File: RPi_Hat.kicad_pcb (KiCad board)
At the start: 2 copper layers, 65 x 56.5 mm, 21 parts, among them IC1 0.96_I2C_OLED, IC2 7406, IC3 I2C LC, J1 RPi_GPIO, SW1 Select, SW2 Up, SW3 Down, SW4 Exit, SW5 Add Disk

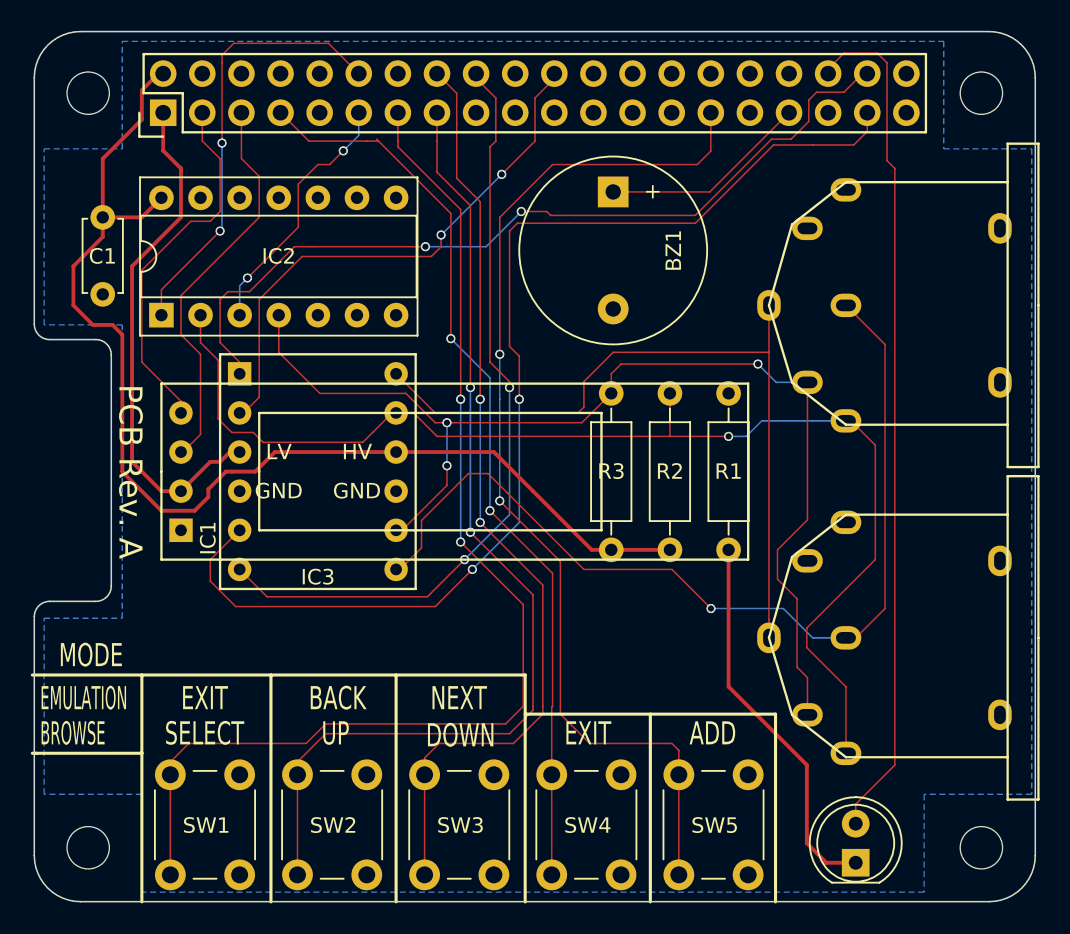
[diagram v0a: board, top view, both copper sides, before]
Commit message: Revision B PCB layout
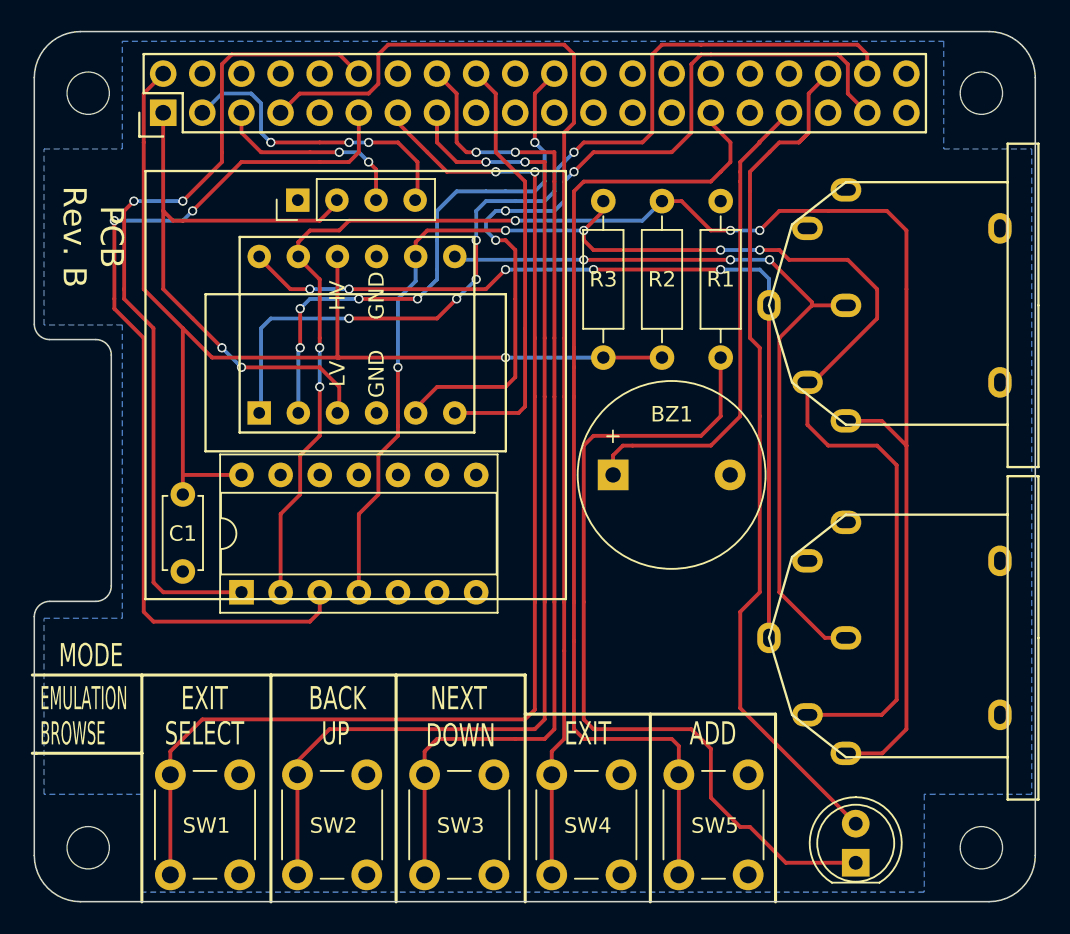
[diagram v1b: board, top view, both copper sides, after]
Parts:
- IC1: footprint IIC_OLED:0.91_I2C_OLED -> IIC_OLED:0.96_I2C_OLED
- IEC_1: renamed from IEC #1
- IEC_2: renamed from IEC #2
- moved IC1 22.0 mm to (43.8, 36.8)
- moved C1 18.7 mm to (33.1, 58.6)
- moved IC2 18.7 mm to (37.0, 65.0)
- moved BZ1 18.4 mm to (61.1, 57.4), turned to 0 degrees
- moved R1 12.5 mm to (68.1, 39.6)
- moved R2 12.5 mm to (64.3, 49.7)
- moved R3 12.5 mm to (60.4, 49.7)
- moved IC3 7.73 mm to (43.2, 48.3), turned to 90 degrees
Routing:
- net RPI_CLK_OUT: track 16.8 -> 60.4 mm
- net Net-(D1-Pad1): track 24.9 -> 54.6 mm
- net C64_DATA: track 78.7 -> 108.4 mm, vias 1 -> 5
- net RPI_DATA_OUT: track 28.5 -> 54.6 mm
- net C64_CLK: track 73.2 -> 98.2 mm, vias 3 -> 5
- net RPI_ATN: track 50.3 -> 27.7 mm, vias 2 -> 0
- net RPI_CLK_IN: track 73.4 -> 54.2 mm, vias 2 -> 3
- net RPI_SND: track 13.5 -> 31.6 mm
- net IN_SW4: track 59.7 -> 77.0 mm, vias 2 -> 0
- net I2C_SCL: track 25.7 -> 13.0 mm, vias 0 -> 2
- net C64_ATN: track 61.3 -> 51.9 mm, vias 1 -> 3
- net C64_RST: track 49.4 -> 58.1 mm, vias 0 -> 5
- net +3V3: track 33.3 -> 39.5 mm, vias 0 -> 2
- net RPI_RST: track 54.5 -> 60.4 mm, vias 2 -> 5
- net +5V: track 76.6 -> 71.3 mm, vias 0 -> 1
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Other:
- board text added: "PCB Rev. B"
- board text removed: "PCB Rev. A"
